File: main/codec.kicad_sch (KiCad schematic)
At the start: 24 parts, among them J1 AudioJack5, U2 TLV320AIC3104IRHBR, U200 AP2120N-1.8TRG1

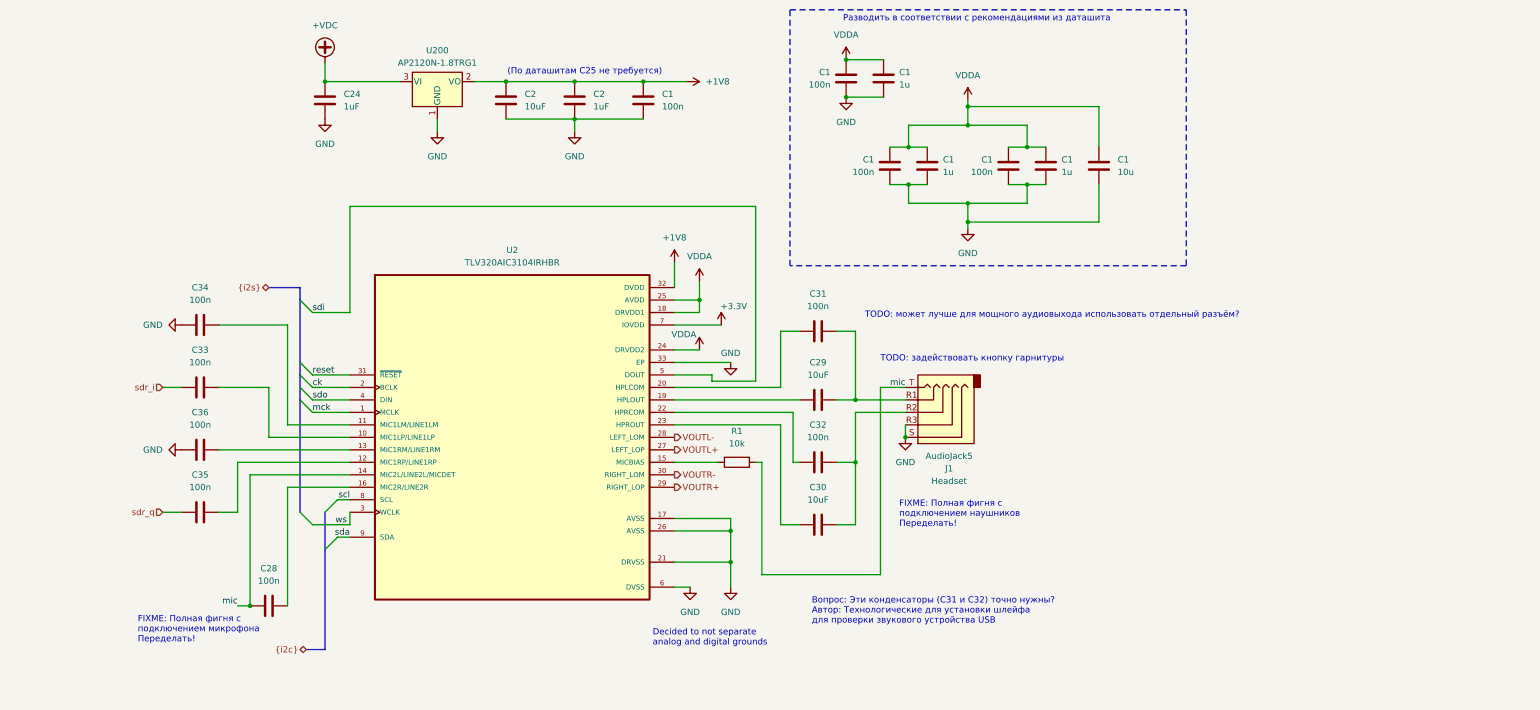
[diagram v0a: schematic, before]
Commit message: Headset layout redrawn, PDF generated
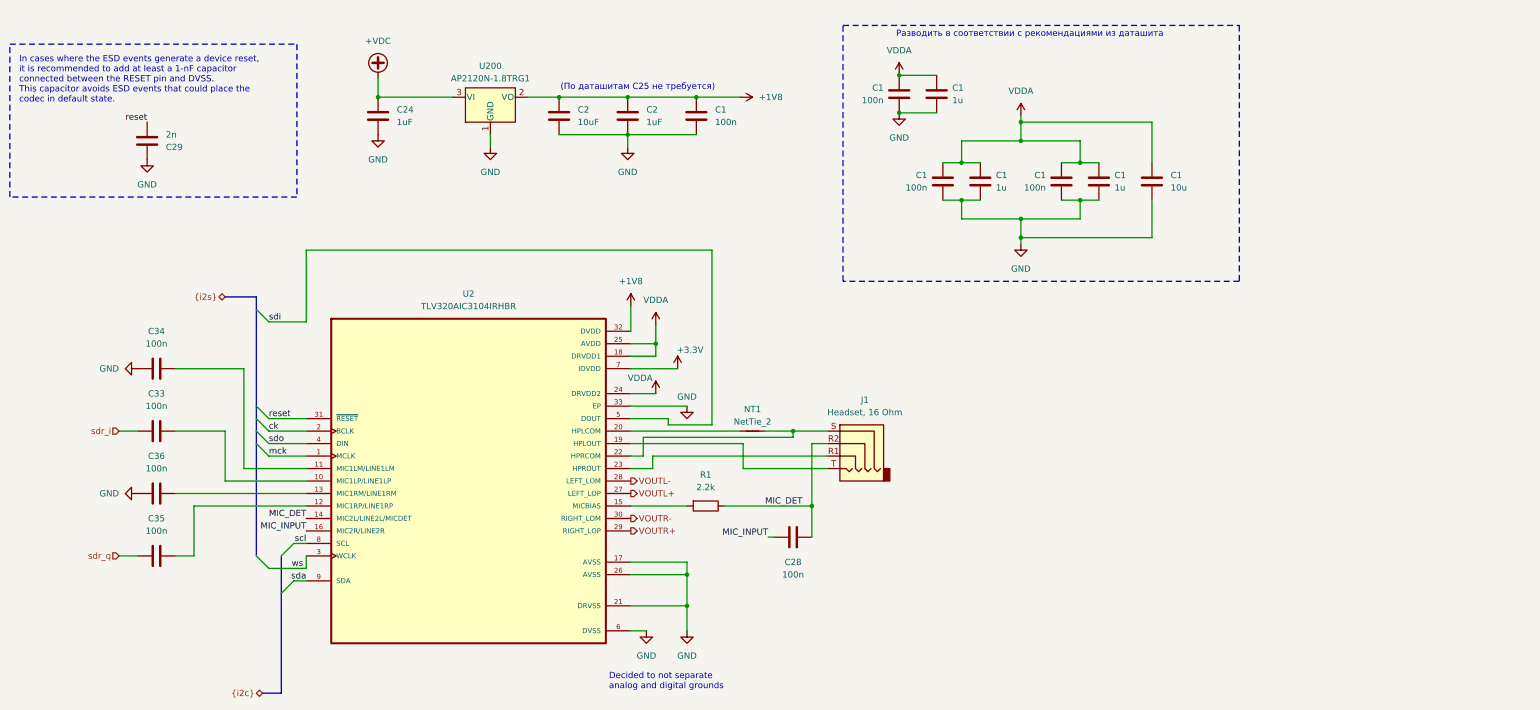
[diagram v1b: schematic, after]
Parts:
- removed C30: 10uF, symbol Device:C
- removed C31, C32: 100n, symbol Device:C
- removed J1: AudioJack5, symbol Connector_Audio:AudioJack5
- added J1: Headset, 16 Ohm, symbol Connector_Audio:AudioJack4
- added NT1: NetTie_2, symbol Device:NetTie_2
- C29: value 10uF -> 2n
- R1: value 10k -> 2.2k
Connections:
- net GND: now also C29.2
- net reset: now also C29.1
- net at U2.20 (HPLCOM): now also NT1.1
- net at U2.23 (HPROUT): now also J1.R1
- net at U2.22 (HPRCOM): now also J1.S, NT1.2
- net MIC_DET: now reaches C28.2
- net MIC_DET: now also R1.1, U2.14 (MIC2L/LINE2L/MICDET), J1.R2; no longer U2.16 (MIC2R/LINE2R)
- net at U2.19 (HPLOUT): now also J1.T; no longer C29.1
- removed net mic: C28.1, R1.1, U2.14 (MIC2L/LINE2L/MICDET)
- new net MIC_INPUT: C28.1, U2.16 (MIC2R/LINE2R)
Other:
- note added: "In cases where the ESD events generate a device reset, it is recommended to add at least a 1-nF capacitor connected between the RESET pin and DVSS. This capacitor avoids ESD events that could place the codec in default state."
- note removed: "FIXME: Полная фигня с подключением микрофона Переделать!"
- note removed: "FIXME: Полная фигня с подключением наушников Переделать!"
- note removed: "TODO: задействовать кнопку гарнитуры"
- note removed: "TODO: может лучше для мощного аудиовыхода использовать отдельный разъём?"
- note removed: "Вопрос: Эти конденсаторы (C31 и C32) точно нужны? Автор: Технологические для установки шлейфа для проверки звукового устройства USB"
- moved on the sheet: C1, C2, C24, C28, C33, C34, C35, C36, R1, U2, U200
